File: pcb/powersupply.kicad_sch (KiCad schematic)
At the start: 19 parts, among them U4 AMS1117-3.3, U5 TPS54302

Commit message: added more part numbers
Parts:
- C57: LCSC (none) -> C4747956; LINK (none) -> https://jlcpcb.com/partdetail/Knscha-RST470UF25V032/C4747956
- C66: LCSC (none) -> C4747956; LINK (none) -> https://jlcpcb.com/partdetail/60989-HV101M010E055ETR/C59937
- D9: LCSC (none) -> C3014033; LINK (none) -> https://jlcpcb.com/partdetail/Fosan-SS54B/C3014033
- U4: LCSC (none) -> C6186; LINK (none) -> https://jlcpcb.com/partdetail/Advanced_MonolithicSystems-AM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
- U5: LCSC (none) -> C311983; LINK (none) -> https://jlcpcb.com/partdetail/TexasInstruments-TPS54302DDCR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
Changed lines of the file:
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@@
+      (effects (font (size 1.27 1.27)) hide)
+    )
+    (property "LCSC" "C311983" (at 99.06 49.53 0)
+      (effects (font (size 1.27 1.27)) hide)
+    )
+    (property "LINK" "https://jlcpcb.com/partdetail/TexasInstruments-TPS54302DDCR/C311983" (at 99.06 49.53 0)
       (effects (font (size 1.27 1.27)) hide)
     )
@@
       (effects (font (size 1.27 1.27)) hide)
     )
+    (property "LCSC" "C4747956" (at 53.34 54.61 0)
+      (effects (font (size 1.27 1.27)) hide)
+    )
+    (property "LINK" "https://jlcpcb.com/partdetail/Knscha-RST470UF25V032/C4747956" (at 53.34 54.61 0)
+      (effects (font (size 1.27 1.27)) hide)
+    )
     (pin "1")
     (pin "2")
@@
       (effects (font (size 1.27 1.27)) hide)
     )
+    (property "LCSC" "C6186" (at 63.5 104.14 0)
+      (effects (font (size 1.27 1.27)) hide)
+    )
+    (property "LINK" "https://jlcpcb.com/partdetail/Advanced_MonolithicSystems-AMS1117_33/C6186" (at 63.5 104.14 0)
+      (effects (font (size 1.27 1.27)) hide)
+    )
     (pin "1")
     (pin "2")
@@
       (effects (font (size 1.27 1.27)) hide)
     )
+    (property "LCSC" "C3014033" (at 39.37 48.26 0)
+      (effects (font (size 1.27 1.27)) hide)
+    )
+    (property "LINK" "https://jlcpcb.com/partdetail/Fosan-SS54B/C3014033" (at 39.37 48.26 0)
+      (effects (font (size 1.27 1.27)) hide)
+    )
     (pin "1")
     (pin "2")
@@
       (effects (font (size 1.27 1.27)) hide)
     )
+    (property "LCSC" "C4747956" (at 85.09 107.95 0)
+      (effects (font (size 1.27 1.27)) hide)
+    )
+    (property "LINK" "https://jlcpcb.com/partdetail/60989-HV101M010E055ETR/C59937" (at 85.09 107.95 0)
+      (effects (font (size 1.27 1.27)) hide)
+    )

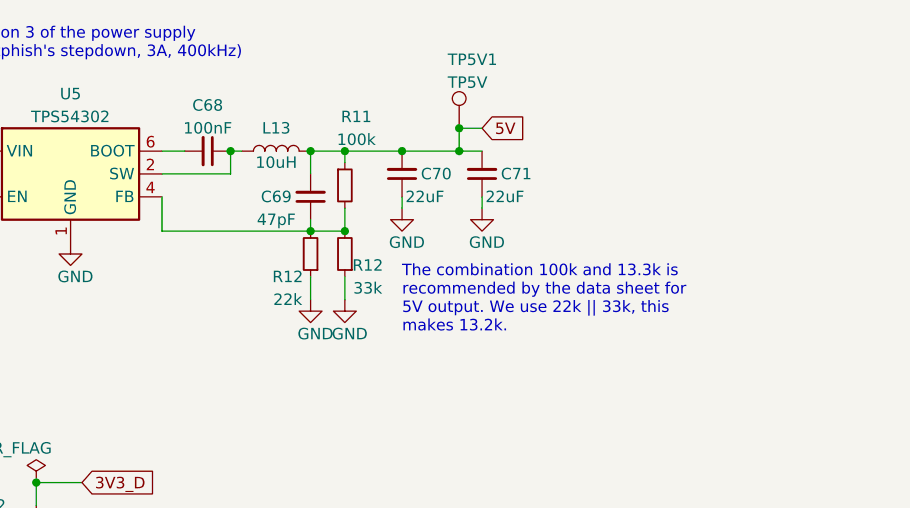
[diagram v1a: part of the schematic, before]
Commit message: more partnumbers assigned. split difficult values into two parts. add protection of CP_SENSE port
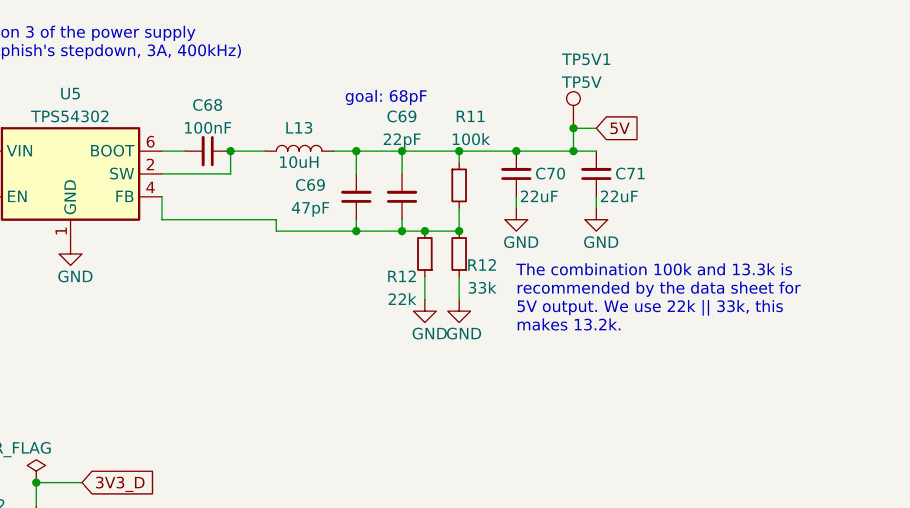
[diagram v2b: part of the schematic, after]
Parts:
- added C69: 22pF, Capacitor_SMD:C_0805_2012Metric_Pad1.18x1.45mm_HandSolder, symbol Device:C_Small
- C66: LCSC C4747956 -> C59937
- R11: footprint Resistor_SMD:R_1206_3216Metric_Pad1.30x1.75mm_HandSolder -> Resistor_SMD:R_0815_2038Metric_Pad1.20x4.05mm_HandSolder; LCSC C25804 -> C149504; LINK (none) -> https://jlcpcb.com/partdetail/160838-0805W8F1003T5E/C149504
- R12: footprint Resistor_SMD:R_1206_3216Metric_Pad1.30x1.75mm_HandSolder -> Resistor_SMD:R_0805_2012Metric_Pad1.20x1.40mm_HandSolder; LCSC C25804 -> C17560; LINK (none) -> https://jlcpcb.com/partdetail/18248-0805W8F2202T5E/C17560
- R12: footprint Resistor_SMD:R_1206_3216Metric_Pad1.30x1.75mm_HandSolder -> Resistor_SMD:R_0815_2038Metric_Pad1.20x4.05mm_HandSolder; LCSC C25804 -> C17633; LINK (none) -> https://jlcpcb.com/partdetail/18321-0805W8F3302T5E/C17633
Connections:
- net 5V: now also C69.2
- net at C69.1, R11.2, R12.2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: now also C69.1
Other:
- note added: "goal: 68pF"
- moved on the sheet: C69, C70, C71, L13, R11, R12, TP5V1

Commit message: footprint corrections. some layout adaptions for new footprints (ongoing)
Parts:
- R11, R12: footprint Resistor_SMD:R_0815_2038Metric_Pad1.20x4.05mm_HandSolder -> Resistor_SMD:R_0805_2012Metric_Pad1.20x1.40mm_HandSolder
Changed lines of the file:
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@@
       (effects (font (size 1.27 1.27)))
     )
-    (property "Footprint" "Resistor_SMD:R_0815_2038Metric_Pad1.20x4.05mm_HandSolder" (at 142.24 50.8 0)
+    (property "Footprint" "Resistor_SMD:R_0805_2012Metric_Pad1.20x1.40mm_HandSolder" (at 142.24 50.8 0)
       (effects (font (size 1.27 1.27)) hide)
     )
@@
       (effects (font (size 1.27 1.27)))
     )
-    (property "Footprint" "Resistor_SMD:R_0815_2038Metric_Pad1.20x4.05mm_HandSolder" (at 142.24 58.42 0)
-      (effects (font (size 1.27 1.27)) hide)
-    )
+    (property "Footprint" "Resistor_SMD:R_0805_2012Metric_Pad1.20x1.40mm_HandSolder" (at 142.24 58.42 0)
+      (effects (font (size 1.27 1.27)) hide)
+    )

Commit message: added part number for the big 10uH
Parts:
- L13: LCSC (none) -> C3000379; LINK (none) -> https://jlcpcb.com/partdetail/3481234-SMDRI125100MT/C3000379
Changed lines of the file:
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@@
       (effects (font (size 1.27 1.27)) hide)
     )
-    (property "Datasheet" "https://datasheet.lcsc.com/lcsc/1810231814_Murata-Electronics-LQM31PN4R7M00L_C162588.pdf" (at 124.46 46.99 0)
+    (property "Datasheet" "~" (at 124.46 46.99 0)
       (effects (font (size 1.27 1.27)) hide)
     )
-    (property "LCSC" "" (at 124.46 46.99 90)
+    (property "LCSC" "C3000379" (at 124.46 46.99 90)
       (effects (font (size 1.27 1.27)) hide)
     )
+    (property "LINK" "https://jlcpcb.com/partdetail/3481234-SMDRI125100MT/C3000379" (at 124.46 46.99 0)
+      (effects (font (size 1.27 1.27)) hide)
+    )

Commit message: added rotation attribute to get the correct footprint rotation at JLCPCB
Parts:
- U4: JLCPCB Rotation Offset (none) -> 180
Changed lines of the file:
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@@
+      (effects (font (size 1.27 1.27)) hide)
+    )
+    (property "JLCPCB Rotation Offset" "180" (at 63.5 104.14 0)
       (effects (font (size 1.27 1.27)) hide)
     )
